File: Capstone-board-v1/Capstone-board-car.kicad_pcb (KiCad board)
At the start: 2 copper layers, 54.1 x 52.8 mm, 26 parts, among them J1 Pcio Socket 1, J2 Pico Socket 2, J3 Ultra Sonic Sensor, J4 Car, J5 Camera, J6 Gyroscope Sensor, U1 3.3V Voltage Regulator, U2 555 Timer, U3 5V Voltage Regulator 2, U4 5V Voltage Regulator 1

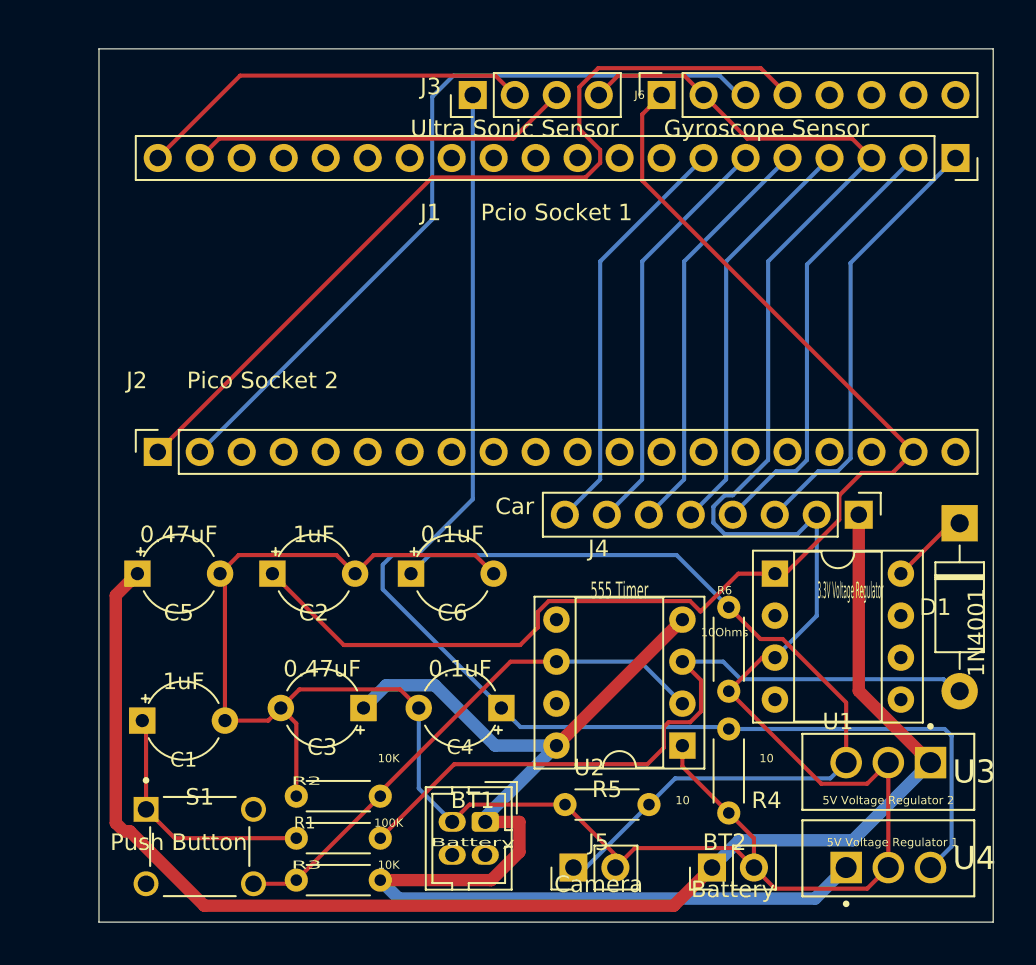
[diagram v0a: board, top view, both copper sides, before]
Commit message: Final PCB completed!
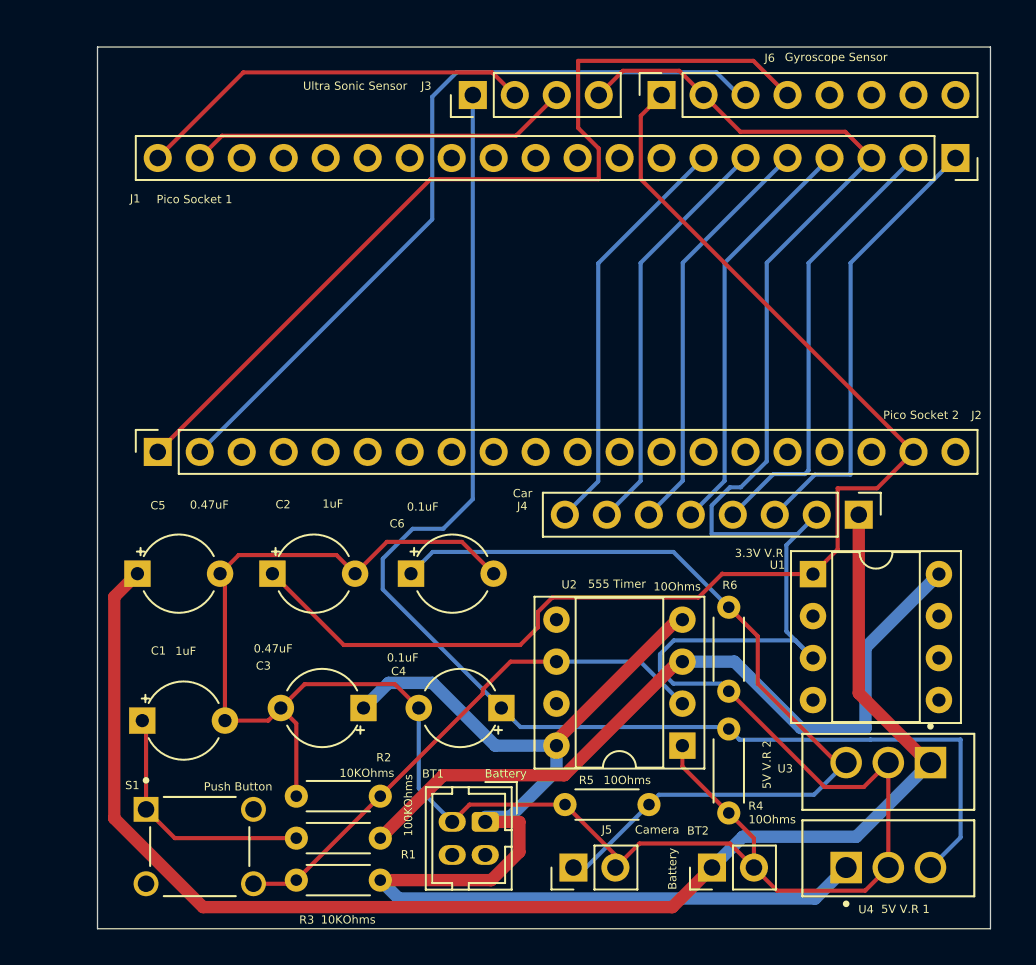
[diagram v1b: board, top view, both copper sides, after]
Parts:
- removed D1: 1N4001, Diode_THT:D_DO-41_SOD81_P10.16mm_Horizontal
- J1: value Pcio Socket 1 -> Pico Socket 1
- R1: value 100K -> 100KOhms
- R2, R3: value 10K -> 10KOhms
- R4, R5: value 10 -> 10Ohms
- U1: value 3.3V Voltage Regulator -> 3.3V V.R
- U3: value 5V Voltage Regulator 2 -> 5V V.R 2
- U4: value 5V Voltage Regulator 1 -> 5V V.R 1
- moved U1 2.30 mm to (79.0, 103.2)
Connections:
- R1 pad 2: Net-(D1-A) -> Net-(U1-IN)
- U1 pad 8: Net-(D1-K) -> Net-(U1-IN)
- U2 pad 3: Net-(D1-A) -> Net-(U1-IN)
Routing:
- net Net-(U1-IN): track 0.00 -> 47.7 mm
- net Net-(D1-A): track 43.7 -> 0.00 mm
- net Earth: track 178.5 -> 191.6 mm
- net Net-(D1-K): track 4.56 -> 0.00 mm
- net Net-(J2-Pin_1): track 52.9 -> 54.7 mm
- net VCC: track 73.4 -> 74.5 mm
- net Net-(J2-Pin_19): track 76.2 -> 77.1 mm
- net Net-(J3-Pin_1): track 79.6 -> 80.5 mm
- net Net-(J1-Pin_1): track 26.8 -> 27.4 mm
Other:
- board size 54.1 x 52.8 mm -> 54 x 53.3 mm

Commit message: Final PCB's done.
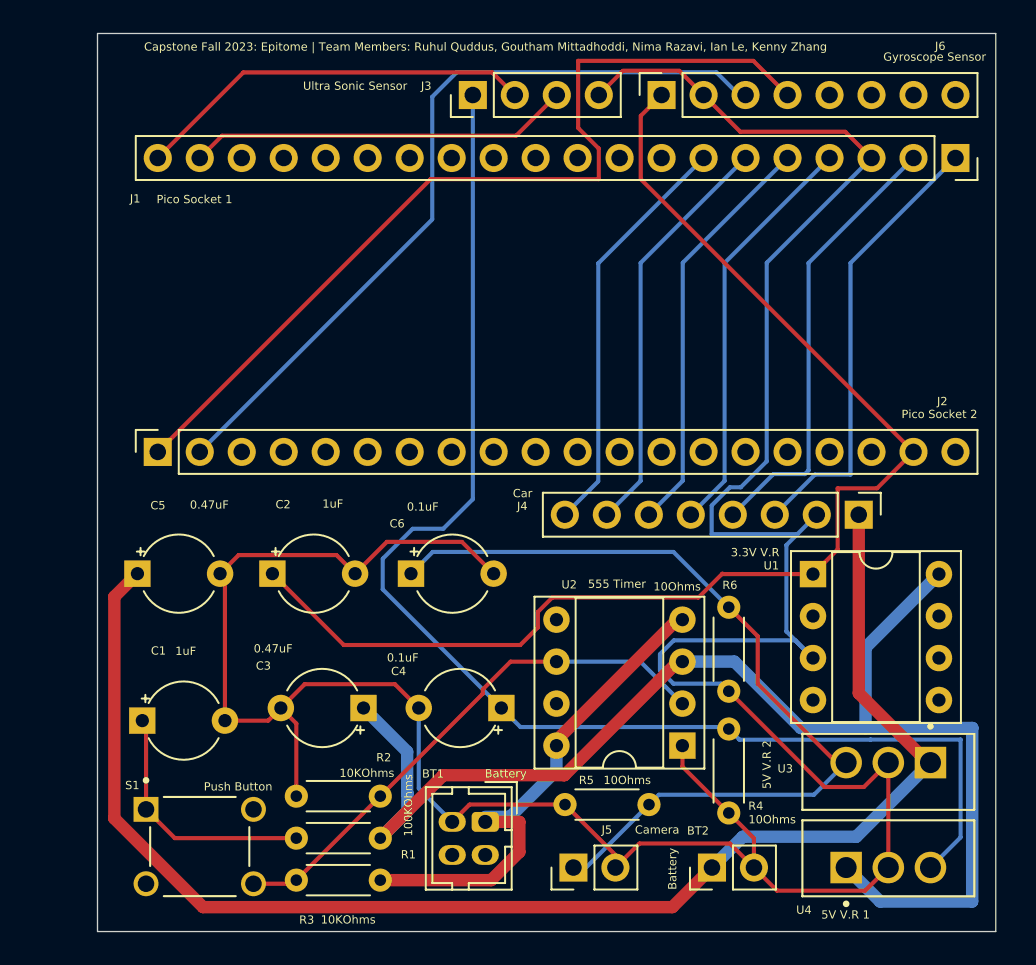
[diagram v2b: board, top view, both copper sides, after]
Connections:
- C3 pad 1: VCC -> Net-(U1-IN)
- U4 pad 1: VCC -> Net-(U1-IN)
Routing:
- net VCC: track 74.5 -> 31.2 mm
- net Net-(U1-IN): track 47.7 -> 82.8 mm
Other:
- board size 54 x 53.3 mm -> 54.3 x 54.3 mm
- board text added: "Capstone Fall 2023: Epitome | Team Members: Ruhul Quddus, Goutham Mittadhoddi, Nima Razavi, Ian Le, Kenny Zhang"
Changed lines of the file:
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@@
     (pad_to_mask_clearance 0)
     (pcbplotparams
-      (layerselection 0x00010fc_ffffffff)
+      (layerselection 0x00010f0_ffffffff)
       (plot_on_all_layers_selection 0x0000000_00000000)
       (disableapertmacros false)
@@
       (outputformat 1)
       (mirror false)
-      (drillshape 1)
+      (drillshape 0)
       (scaleselection 1)
-      (outputdirectory "")
+      (outputdirectory "C:/Users/ruhul/OneDrive/Desktop/Capstone/capstone-project/Car PCB Gerber Files/")
     )
   )
@@
     (property "ki_keywords" "LT1121CN8#PBF")
     (attr through_hole)
-    (fp_text reference "U1" (at -2.148 -0.554) (layer "F.SilkS")
-        (effects (font (size 0.5 0.5) (thickness 0.125)))
-    )
-    (fp_text value "3.3V V.R" (at -3.258 -1.264) (layer "F.SilkS")
+    (fp_text reference "U1" (at -2.52 -0.51) (layer "F.SilkS")
+        (effects (font (size 0.5 0.5) (thickness 0.125)))
+    )
+    (fp_text value "3.3V V.R" (at -3.5 -1.31) (layer "F.SilkS")
         (effects (font (size 0.5 0.5) (thickness 0.125)))
     )
@@
     (fp_line (start 4 3.5) (end 4 -1.5)
       (stroke (width 0.1) (type solid)) (layer "F.Fab"))
-    (pad "1" thru_hole roundrect (at 0 0 270) (size 1.2 1.65) (drill 0.85) (layers "*.Cu" "*.Mask") (roundrect_rratio 0.208333)
+    (pad "1" thru_hole roundrect (at 0 0 270) (size 1.2 1.65) (drill 0.85) (layers "*.Cu" "*.Mask") (roundrect_rratio 0.2083333333)
       (net 1 "VCC") (pinfunction "+") (pintype "passive"))
     (pad "2" thru_hole oval (at 0 2 270) (size 1.2 1.65) (drill 0.85) (layers "*.Cu" "*.Mask")
@@
     (property "ki_keywords" "Voltage Regulator 1.5A Positive")
     (attr through_hole)
-    (fp_text reference "U4" (at 1.204 2.536) (layer "F.SilkS")
-        (effects (font (size 0.5 0.5) (thickness 0.125)))
-    )
-    (fp_text value "5V V.R 1" (at 3.584 2.516) (layer "F.SilkS")
+    (fp_text reference "U4" (at -2.556 2.566) (layer "F.SilkS")
+        (effects (font (size 0.5 0.5) (thickness 0.125)))
+    )
+    (fp_text value "5V V.R 1" (at -0.036 2.856) (layer "F.SilkS")
         (effects (font (size 0.5 0.5) (thickness 0.125)))
     )
@@
       (stroke (width 0.2) (type solid)) (fill none) (layer "F.Fab"))
     (pad "1" thru_hole rect (at 0 0) (size 1.91 1.91) (drill 1.27) (layers "*.Cu" "*.Mask")
-      (net 1 "VCC") (pinfunction "IN") (pintype "power_in") (solder_mask_margin 0.102))
+      (net 8 "Net-(U1-IN)") (pinfunction "IN") (pintype "power_in") (solder_mask_margin 0.102))
     (pad "2" thru_hole circle (at 2.55 0) (size 1.91 1.91) (drill 1.27) (layers "*.Cu" "*.Mask")
       (net 2 "Earth") (pinfunction "GND") (pintype "power_in") (solder_mask_margin 0.102))
@@
     (property "ki_keywords" "connector")
     (attr through_hole)
-    (fp_text reference "J2" (at 2.218 49.53 180) (layer "F.SilkS")
-        (effects (font (size 0.5 0.5) (thickness 0.125)))
-    )
-    (fp_text value "Pico Socket 2" (at 2.228 46.18 180) (layer "F.SilkS")
+    (fp_text reference "J2" (at 3.058 47.46 180) (layer "F.SilkS")
+        (effects (font (size 0.5 0.5) (thickness 0.125)))
+    )
+    (fp_text value "Pico Socket 2" (at 2.278 47.29 180) (layer "F.SilkS")
         (effects (font (size 0.5 0.5) (thickness 0.125)))
     )
@@
         (effects (font (size 0.5 0.5) (thickness 0.125)))
     )
-    (fp_text value "Gyroscope Sensor" (at 2.288 10.56 180) (layer "F.SilkS")
-        (effects (font (size 0.5 0.5) (thickness 0.125)))
-    )
-    (fp_text user "${REFERENCE}" (at 2.238 6.54) (layer "F.SilkS")
+    (fp_text value "Gyroscope Sensor" (at 2.308 16.52 180) (layer "F.SilkS")
+        (effects (font (size 0.5 0.5) (thickness 0.125)))
+    )
+    (fp_text user "${REFERENCE}" (at 2.958 16.86) (layer "F.SilkS")
         (effects (font (size 0.5 0.5) (thickness 0.125)))
     )
@@
       (stroke (width 0.1) (type solid)) (fill none) (layer "F.Fab"))
     (pad "1" thru_hole rect (at 0 0 180) (size 1.6 1.6) (drill 0.8) (layers "*.Cu" "*.Mask")
-      (net 1 "VCC") (pintype "passive"))
+      (net 8 "Net-(U1-IN)") (pintype "passive"))
     (pad "2" thru_hole circle (at 5 0 180) (size 1.6 1.6) (drill 0.8) (layers "*.Cu" "*.Mask")
       (net 2 "Earth") (pintype "passive"))
@@
     )
   )
-  (gr_rect (start 35.724 71.264) (end 89.746 124.606)
+  (gr_rect (start 35.724 70.444) (end 90.066 124.776)
     (stroke (width 0.05) (type default)) (fill none) (layer "Edge.Cuts"))
+  (gr_text "Capstone Fall 2023: Epitome | Team Members: Ruhul Quddus, Goutham Mittadhoddi, Nima Razavi, Ian Le, Kenny Zhang\n" (at 59.2 71.25) (layer "F.SilkS")
+    (effects (font (size 0.5 0.5) (thickness 0.125)))
+  )
+  (dimension (type aligned) (layer "B.Cu")
+    (pts (xy 90.066 124.776) (xy 90.066 70.444))
+    (height 14.134)
+    (gr_text "54.3320 mm" (at 102.4 97.61 90) (layer "B.Cu")
+      (effects (font (size 1.5 1.5) (thickness 0.3)))
+    )
+    (format (prefix "") (suffix "") (units 3) (units_format 1) (precision 4))
+    (style (thickness 0.2) (arrow_length 1.27) (text_position_mode 0) (extension_height 0.58642) (extension_offset 0.5) keep_text_aligned)
+  )
+  (dimension (type aligned) (layer "B.Cu")
+    (pts (xy 35.724 124.776) (xy 90.066 124.776))
+    (height 5.034)
+    (gr_text "54.3420 mm" (at 62.895 128.01) (layer "B.Cu")
+      (effects (font (size 1.5 1.5) (thickness 0.3)))
+    )
+    (format (prefix "") (suffix "") (units 3) (units_format 1) (precision 4))
+    (style (thickness 0.2) (arrow_length 1.27) (text_position_mode 0) (extension_height 0.58642) (extension_offset 0.5) keep_text_aligned)
+  )
   (segment (start 59.182 118.142) (end 61.246 118.142) (width 0.75) (layer "F.Cu") (net 1))
   (segment (start 63.49 113.21) (end 63.49 113.528) (width 0.75) (layer "F.Cu") (net 1))
@@
   (segment (start 60.684 117.836) (end 63.49 115.03) (width 0.75) (layer "B.Cu") (net 1))
   (segment (start 63.49 115.03) (end 63.49 113.528) (width 0.75) (layer "B.Cu") (net 1))
-  (segment (start 53.338 109.73) (end 55.991 109.73) (width 0.75) (layer "B.Cu") (net 1))
-  (segment (start 59.789 113.528) (end 63.49 113.528) (width 0.75) (layer "B.Cu") (net 1))
-  (segment (start 55.991 109.73) (end 59.789 113.528) (width 0.75) (layer "B.Cu") (net 1))
-  (segment (start 79.141 122.779) (end 53.945 122.779) (width 0.75) (layer "B.Cu") (net 1))
-  (segment (start 53.945 122.779) (end 52.832 121.666) (width 0.75) (layer "B.Cu") (net 1))
-  (segment (start 51.816 111.252) (end 53.338 109.73) (width 0.75) (layer "B.Cu") (net 1))
-  (segment (start 81.016 120.904) (end 79.141 122.779) (width 0.75) (layer "B.Cu") (net 1))
   (segment (start 59.182 118.142) (end 59.182 117.836) (width 0.25) (layer "B.Cu") (net 1))
   (segment (start 64.008 117.094) (end 67.056 120.142) (width 0.25) (layer "F.Cu") (net 2))
@@
   (segment (start 52.832 119.126) (end 53.166 119.46) (width 0.25) (layer "F.Cu") (net 8))
   (segment (start 56.638 115.32) (end 52.832 119.126) (width 0.75) (layer "F.Cu") (net 8))
+  (segment (start 88.65 112.46) (end 82.2 112.46) (width 0.75) (layer "B.Cu") (net 8))
+  (segment (start 54.458 116.407949) (end 54.47 116.419949) (width 0.75) (layer "B.Cu") (net 8))
+  (segment (start 88.64 112.47) (end 88.65 112.46) (width 0.75) (layer "B.Cu") (net 8))
+  (segment (start 81.016 120.904) (end 83.072 122.96) (width 0.75) (layer "B.Cu") (net 8))
   (segment (start 78.28 112.47) (end 74.258 108.448) (width 0.75) (layer "B.Cu") (net 8))
+  (segment (start 88.64 122.96) (end 88.64 112.47) (width 0.75) (layer "B.Cu") (net 8))
+  (segment (start 82.2 112.46) (end 82.19 112.47) (width 0.75) (layer "B.Cu") (net 8))
+  (segment (start 83.072 122.96) (end 88.64 122.96) (width 0.75) (layer "B.Cu") (net 8))
   (segment (start 82.19 107.59) (end 82.19 112.47) (width 0.75) (layer "B.Cu") (net 8))
   (segment (start 86.63 103.15) (end 82.19 107.59) (width 0.75) (layer "B.Cu") (net 8))
+  (segment (start 54.47 117.488) (end 52.832 119.126) (width 0.75) (layer "B.Cu") (net 8))
+  (segment (start 51.816 111.252) (end 54.458 113.894) (width 0.75) (layer "B.Cu") (net 8))
   (segment (start 71.11 109.08) (end 71.11 108.448) (width 0.25) (layer "B.Cu") (net 8))
   (segment (start 82.19 112.47) (end 78.28 112.47) (width 0.75) (layer "B.Cu") (net 8))
   (segment (start 74.258 108.448) (end 71.11 108.448) (width 0.75) (layer "B.Cu") (net 8))
+  (segment (start 54.47 116.419949) (end 54.47 117.488) (width 0.75) (layer "B.Cu") (net 8))
+  (segment (start 54.458 113.894) (end 54.458 116.407949) (width 0.75) (layer "B.Cu") (net 8))
   (segment (start 79.126 97.13) (end 81.28 97.13) (width 0.25) (layer "B.Cu") (net 9))
   (segment (start 76.698 99.558) (end 79.126 97.13) (width 0.25) (layer "B.Cu") (net 9))
